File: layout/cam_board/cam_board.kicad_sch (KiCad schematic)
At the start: 46 parts, among them J1 Debug, J2 USB Connector, J3 BATT_CONNECTOR, SW1 SW_MEC_5E, SW2 SW_MEC_5E, SW3 SW_MEC_5E, SW4 PWR, U1 STM32F401CCUx, U2 USBLC6-2SC6, U3 LD1117S33TR_SOT223, U4 MCP73831-2-OT, Y1 ECS-80-18-23B-JTN-TR, Y2 SC32S-7PF20PPM

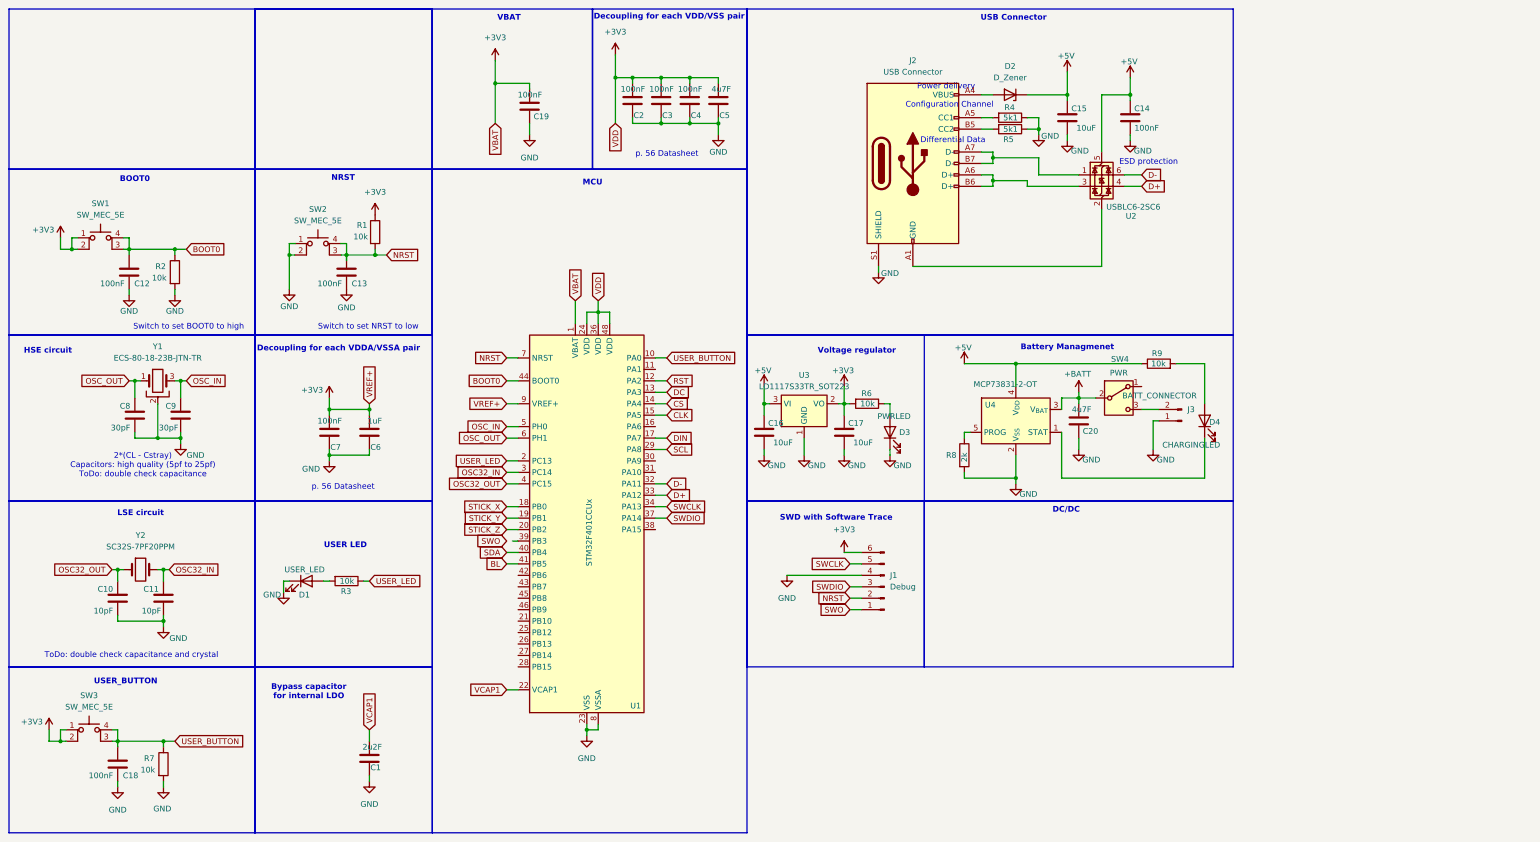
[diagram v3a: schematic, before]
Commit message: Update layout and schematic
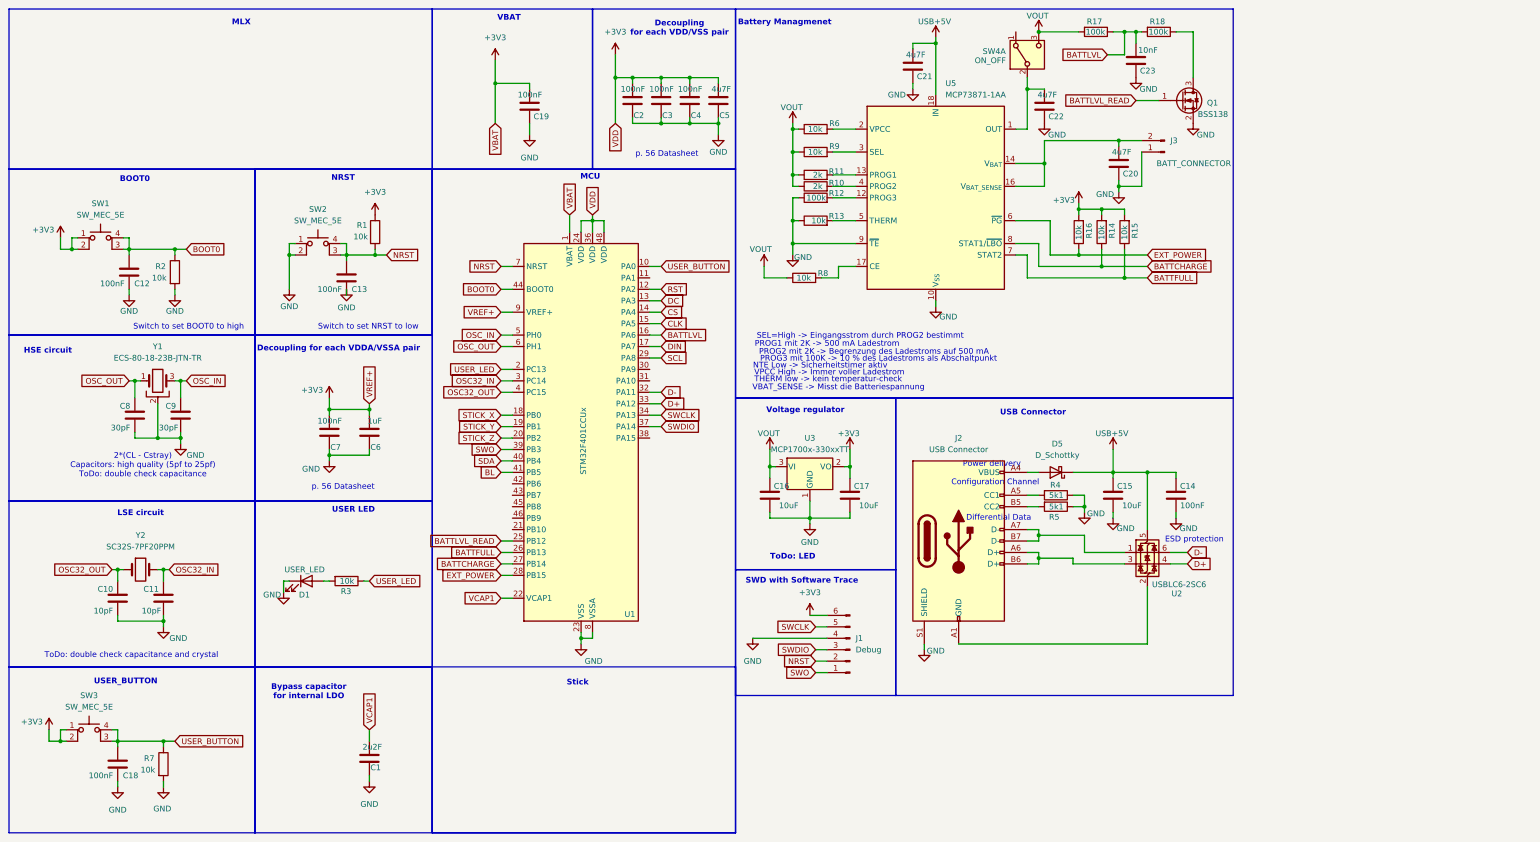
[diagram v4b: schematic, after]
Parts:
- removed D2: D_Zener, Diode_SMD:D_0201_0603Metric_Pad0.64x0.40mm_HandSolder, symbol Device:D_Zener
- removed D3: PWRLED, LED_SMD:LED_0603_1608Metric_Pad1.05x0.95mm_HandSolder, symbol Device:LED
- removed D4: CHARGINGLED, LED_SMD:LED_0603_1608Metric_Pad1.05x0.95mm_HandSolder, symbol Device:LED
- removed SW4: PWR, symbol Switch:SW_SPDT
- removed U3: LD1117S33TR_SOT223, Package_TO_SOT_SMD:SOT-223-3_TabPin2, symbol Regulator_Linear:LD1117S33TR_SOT223
- removed U4: MCP73831-2-OT, Package_TO_SOT_SMD:SOT-23-5_HandSoldering, symbol Battery_Management:MCP73831-2-OT
- added C21, C22: 4u7F, Capacitor_SMD:C_0603_1608Metric_Pad1.08x0.95mm_HandSolder, symbol Device:C
- added C23: 10nF, Capacitor_SMD:C_0603_1608Metric_Pad1.08x0.95mm_HandSolder, symbol Device:C
- added D5: D_Schottky, Diode_SMD:D_0603_1608Metric_Pad1.05x0.95mm_HandSolder, symbol Device:D_Schottky
- added Q1: BSS138, Package_TO_SOT_SMD:SOT-23_Handsoldering, symbol Transistor_FET:BSS138
- added R10, R11: 2k, Resistor_SMD:R_0603_1608Metric_Pad0.98x0.95mm_HandSolder, symbol Device:R
- added R12, R17, R18: 100k, Resistor_SMD:R_0603_1608Metric_Pad0.98x0.95mm_HandSolder, symbol Device:R
- added R13, R14, R15, R16: 10k, Resistor_SMD:R_0603_1608Metric_Pad0.98x0.95mm_HandSolder, symbol Device:R
- added SW4: ON_OFF, symbol Switch:SW_DPDT_x2
- added U3: MCP1700x-330xxTT, Package_TO_SOT_SMD:SOT-23_Handsoldering, symbol Regulator_Linear:MCP1700x-330xxTT
- added U5: MCP73871-1AA, Package_DFN_QFN:QFN-20-1EP_4x4mm_P0.5mm_EP2.5x2.5mm_ThermalVias, symbol Battery_Management:MCP73871-1AA
- R8: value 2k -> 10k
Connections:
- net +BATT is gone; now on an unnamed net: C20.2
- net +3V3: now also R14.2, R15.2, R16.2, U3.2 (VO); no longer R6.2
- net GND: now also C21.1, C22.1, C23.1, Q1.2 (S), R12.1, R13.1, U3.1 (GND), U5.10 (V_{SS}), U5.11 (V_{SS}), U5.21 (V_{SS}), U5.9 (~{TE}); no longer R8.2
- net SWO: now also U1.39 (PB3)
- net at R9.2: now also U5.3 (SEL)
- net at J3.2 (Pin_2): now also U5.14 (V_{BAT}), U5.15 (V_{BAT}), U5.16 (V_{BAT_SENSE})
- net at J2.A4 (VBUS), J2.A9 (VBUS), J2.B4 (VBUS)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: now also D5.2 (A)
- net BATTLVL: now reaches U1.16 (PA6)
- net BATTLVL: now also C23.2, R17.1, R18.2
- net BATTLVL_READ: now reaches U1.25 (PB12)
- net BATTLVL_READ: now also Q1.1 (G)
- net BATTFULL: now reaches U1.26 (PB13)
- net BATTFULL: now also R15.1, U5.7 (STAT2)
- net BATTCHARGE: now reaches U1.27 (PB14)
- net BATTCHARGE: now also R14.1, U5.8 (STAT1/~{LBO})
- net EXT_POWER: now reaches U1.28 (PB15)
- net EXT_POWER: now also R16.1, U5.6 (~{PG})
- net VOUT: now reaches R8.1
- net VOUT: now also C16.2, R6.1, R9.1, R10.1, R11.1, R17.2, SW4.3 (C), U3.3 (VI)
- net +5V renamed USB+5V
- net USB+5V: now also C21.2, D5.1 (K), U5.18 (IN), U5.19 (IN); no longer C16.2, R9.1
- new net: R10.2, U5.4 (PROG2)
- new net: R6.2, U5.2 (VPCC)
- new net: R11.2, U5.13 (PROG1)
- new net: R13.2, U5.5 (THERM)
- new net: C22.2, SW4.2 (B), U5.1 (OUT), U5.20 (OUT)
- new net: Q1.3 (D), R18.1
- new net: R12.2, U5.12 (PROG3)
- new net: R8.2, U5.17 (CE)
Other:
- note added: "MLX"
- note added: "NTE Low -> Sicherheitstimer aktiv"
- note added: "PROG1 mit 2K -> 500 mA Ladestrom"
- note added: "PROG2 mit 2K -> Begrenzung des Ladestroms auf 500 mA"
- note added: "PROG3 mit 100K -> 10 % des Ladestroms als Abschaltpunkt"
- note added: "SEL=High -> Eingangsstrom durch PROG2 bestimmt"
- note added: "Stick"
- note added: "THERM low -> kein temperatur-check"
- note added: "ToDo: LED"
- note added: "VBAT_SENSE -> Misst die Batteriespannung"
- note added: "VPCC High -> Immer voller Ladestrom"
- note removed: "DC/DC"
- moved on the sheet: C13, C14, C15, C16, C17, C20, J1, J2, J3, R4, R5, U1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

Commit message: First full schematic
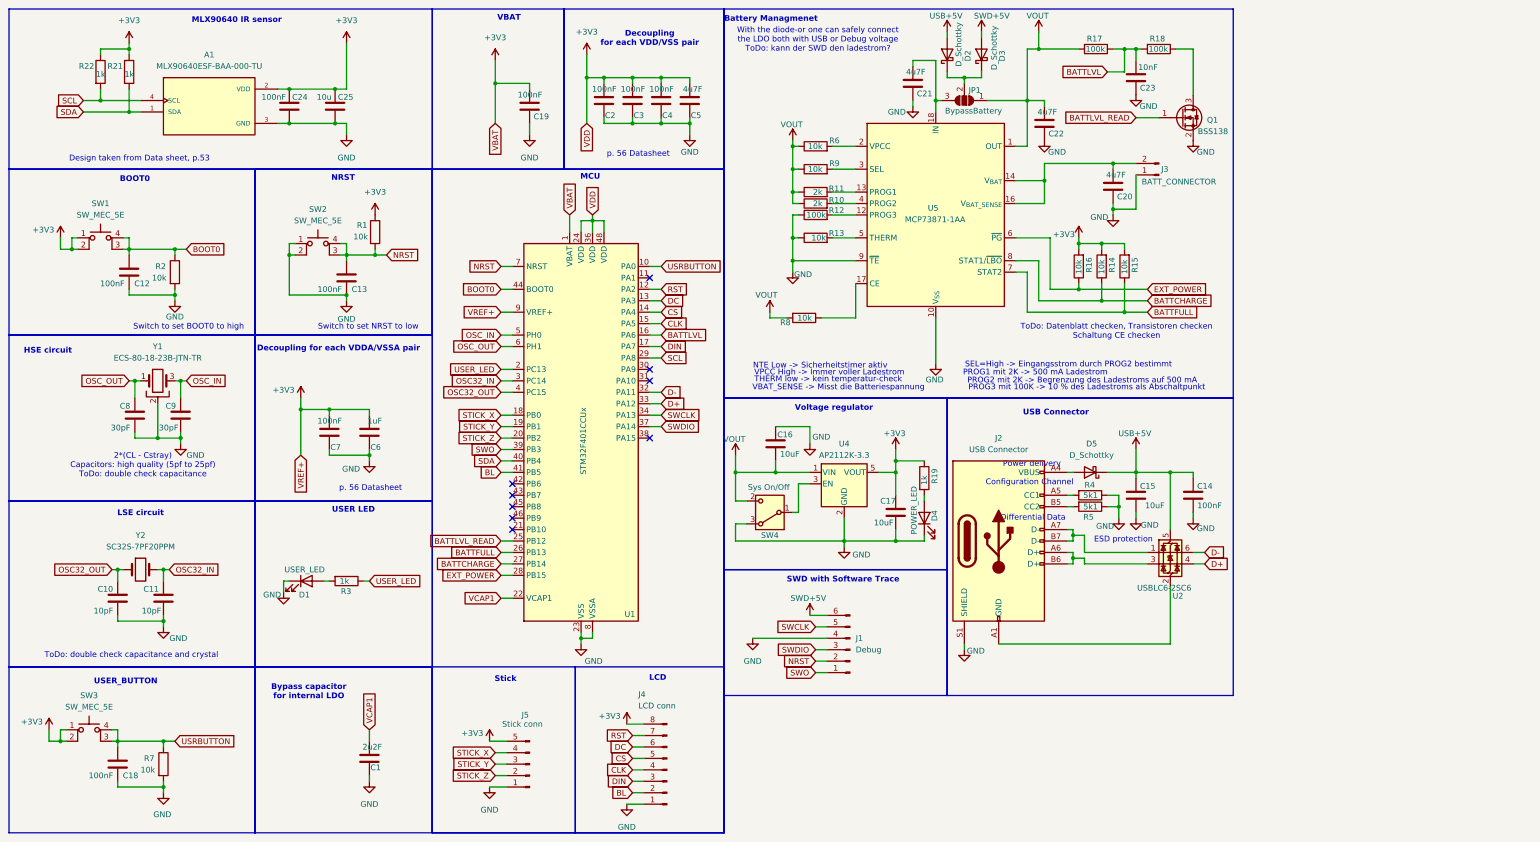
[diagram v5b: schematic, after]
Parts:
- removed SW4: ON_OFF, symbol Switch:SW_DPDT_x2
- removed U3: MCP1700x-330xxTT, Package_TO_SOT_SMD:SOT-23_Handsoldering, symbol Regulator_Linear:MCP1700x-330xxTT
- added A1: MLX90640ESF-BAA-000-TU, A_Custom:TO292P930H600-4-MLX, symbol Custom:MLX90640ESF-BAA-000-TU
- added C24: 100nF, Capacitor_SMD:C_0603_1608Metric_Pad1.08x0.95mm_HandSolder, symbol Device:C
- added C25: 10u, Capacitor_SMD:C_0603_1608Metric_Pad1.08x0.95mm_HandSolder, symbol Device:C
- added D2, D3: D_Schottky, Diode_SMD:D_0603_1608Metric_Pad1.05x0.95mm_HandSolder, symbol Device:D_Schottky
- added D4: POWER_LED, LED_SMD:LED_0603_1608Metric_Pad1.05x0.95mm_HandSolder, symbol Device:LED
- added J4: LCD conn, Connector_PinHeader_1.27mm:PinHeader_1x08_P1.27mm_Vertical, symbol Connector:Conn_01x08_Pin
- added J5: Stick conn, Connector_PinHeader_1.27mm:PinHeader_1x05_P1.27mm_Vertical, symbol Connector:Conn_01x05_Pin
- added JP1: BypassBattery, Jumper:SolderJumper-3_P1.3mm_Open_RoundedPad1.0x1.5mm_NumberLabels, symbol Jumper:SolderJumper_3_Open
- added R19, R21, R22: 1k, Resistor_SMD:R_0603_1608Metric_Pad0.98x0.95mm_HandSolder, symbol Device:R
- added SW4: Sys On/Off, Button_Switch_SMD:SW_DIP_SPSTx01_Slide_6.7x4.1mm_W6.73mm_P2.54mm_LowProfile_JPin, symbol Switch:SW_SPDT_312
- added U4: AP2112K-3.3, Package_TO_SOT_SMD:SOT-23-5_HandSoldering, symbol Regulator_Linear:AP2112K-3.3
- J1: footprint (none) -> Connector_PinHeader_1.27mm:PinHeader_1x06_P1.27mm_Vertical
- J2: footprint (none) -> Connector_USB:USB_C_Receptacle_HRO_TYPE-C-31-M-12
- J3: footprint (none) -> Connector_JST:JST_PH_B2B-PH-K_1x02_P2.00mm_Vertical
- R3: value 10k -> 1k
- Y1: footprint (none) -> A_Custom:XTAL_ECS-80-18-23B-JTN-TR
- Y2: footprint (none) -> A_Custom:XTAL_CM8V-T1A-32.768KHZ-6PF-20PPM-TA-QC
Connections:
- net +3V3: now also A1.2 (VDD), C24.2, C25.2, J4.8 (Pin_8), J5.5 (Pin_5), R19.1, R21.1, R22.1, U4.5 (VOUT); no longer J1.6 (Pin_6)
- net BL: now also J4.2 (Pin_2)
- net CLK: now also J4.4 (Pin_4)
- net CS: now also J4.5 (Pin_5)
- net DC: now also J4.6 (Pin_6)
- net DIN: now also J4.3 (Pin_3)
- net GND: now also C16.2, A1.3 (GND), C24.1, C25.1, D4.1 (K), J4.1 (Pin_1), J5.1 (Pin_1), SW4.3 (A), U4.2 (GND); no longer C16.1
- net RST: now also J4.7 (Pin_7)
- net SCL: now also A1.4 (SCL), R22.2
- net SDA: now also A1.1 (SDA), R21.2
- net STICK_X: now also J5.4 (Pin_4)
- net STICK_Y: now also J5.3 (Pin_3)
- net STICK_Z: now also J5.2 (Pin_2)
- net USB+5V: now also D2.2 (A); no longer C21.2, U5.18 (IN), U5.19 (IN)
- net VOUT: now also C16.1, C22.2, R8.2, U5.1 (OUT), U5.20 (OUT), JP1.1 (A), SW4.2 (C), U4.1 (VIN); no longer C16.2, R8.1
- net at U5.17 (CE): now also R8.1; no longer R8.2
- net USER_BUTTON renamed USRBUTTON
- new net: D2.1 (K), D3.1 (K), JP1.2 (C)
- new net: C21.2, JP1.3 (B), U5.18 (IN), U5.19 (IN)
- new net: D4.2 (A), R19.2
- new net: SW4.1 (B), U4.3 (EN)
- new net SWD+5V: D3.2 (A), J1.6 (Pin_6)
- no-connect marks 0 -> 9
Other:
- note added: "Design taken from Data sheet, p.53"
- note added: "LCD"
- note added: "MLX90640 IR sensor"
- note added: "ToDo: Datenblatt checken, Transistoren checken Schaltung CE checken"
- note added: "With the diode-or one can safely connect the LDO both with USB or Debug voltage ToDo: kann der SWD den ladestrom?"
- note removed: "MLX"
- note removed: "ToDo: LED"
- moved on the sheet: C14, C15, C16, C17, C2, C20, C21, C22, C23, C3, C4, C5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

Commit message: Update layout and schematic
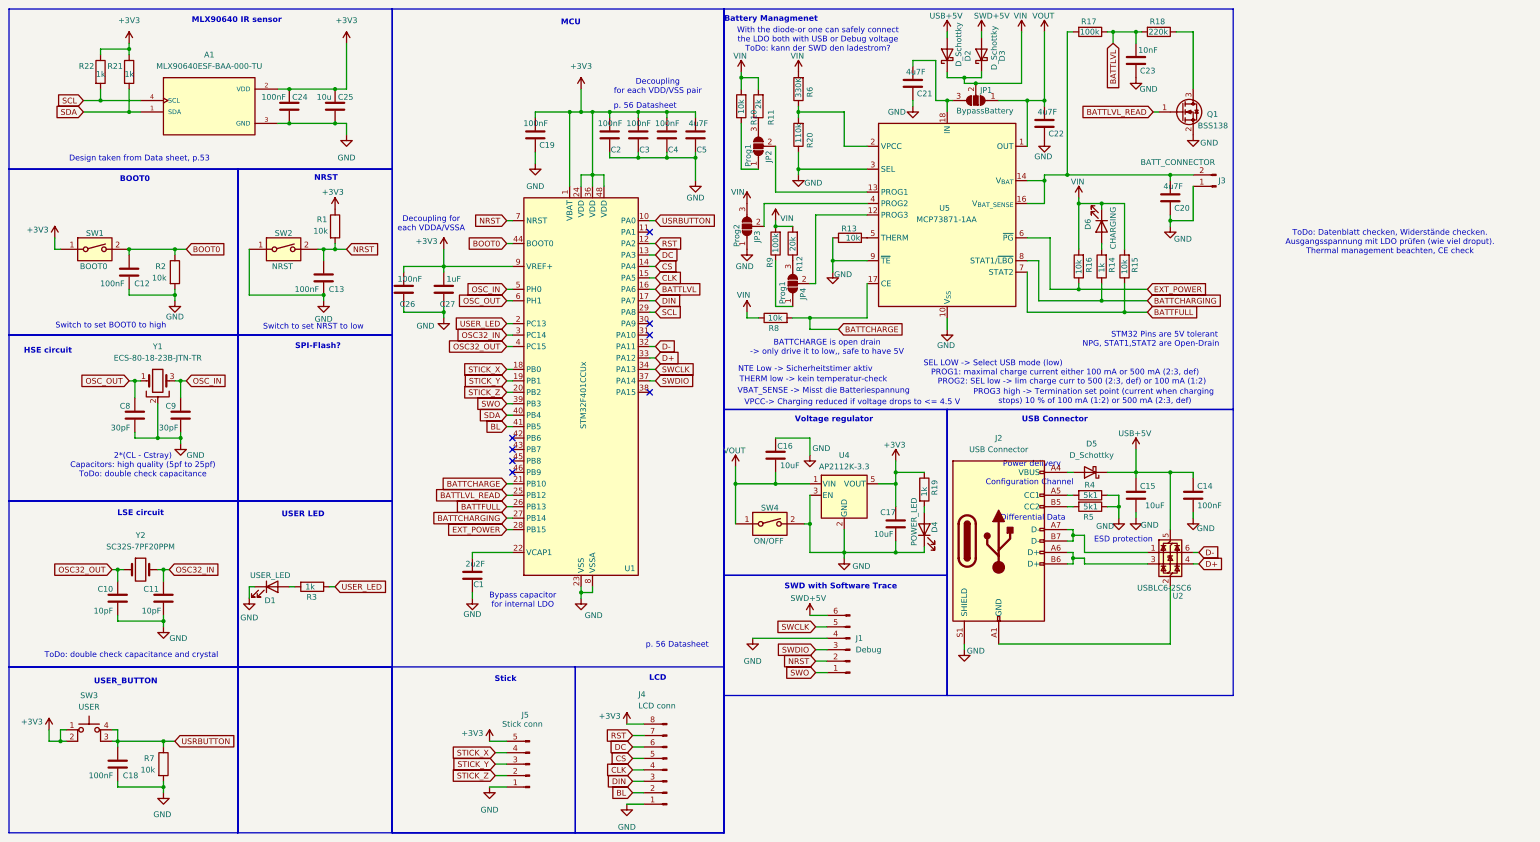
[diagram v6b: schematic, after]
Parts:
- removed C6: 1uF, Capacitor_SMD:C_0603_1608Metric_Pad1.08x0.95mm_HandSolder, symbol Device:C
- removed C7: 100nF, Capacitor_SMD:C_0603_1608Metric_Pad1.08x0.95mm_HandSolder, symbol Device:C
- removed SW1, SW2: SW_MEC_5E, Button_Switch_SMD:SW_MEC_5GSH9, symbol Switch:SW_MEC_5E
- removed SW4: Sys On/Off, Button_Switch_SMD:SW_DIP_SPSTx01_Slide_6.7x4.1mm_W6.73mm_P2.54mm_LowProfile_JPin, symbol Switch:SW_SPDT_312
- added C26: 100nF, Capacitor_SMD:C_0402_1005Metric_Pad0.74x0.62mm_HandSolder, symbol Device:C
- added C27: 1uF, Capacitor_SMD:C_0402_1005Metric_Pad0.74x0.62mm_HandSolder, symbol Device:C
- added D6: CHARGING, LED_SMD:LED_0603_1608Metric_Pad1.05x0.95mm_HandSolder, symbol Device:LED
- added JP2, JP4: Prog1, Jumper:SolderJumper-3_P1.3mm_Open_RoundedPad1.0x1.5mm_NumberLabels, symbol Jumper:SolderJumper_3_Open
- added JP3: Prog2, Jumper:SolderJumper-3_P1.3mm_Open_RoundedPad1.0x1.5mm_NumberLabels, symbol Jumper:SolderJumper_3_Open
- added R20: 110k, Resistor_SMD:R_0603_1608Metric_Pad0.98x0.95mm_HandSolder, symbol Device:R
- added SW1: BOOT0, Button_Switch_SMD:SW_DIP_SPSTx01_Slide_9.78x4.72mm_W8.61mm_P2.54mm, symbol Switch:SW_DIP_x01
- added SW2: NRST, Button_Switch_SMD:SW_DIP_SPSTx01_Slide_9.78x4.72mm_W8.61mm_P2.54mm, symbol Switch:SW_DIP_x01
- added SW4: ON/OFF, Button_Switch_SMD:SW_DIP_SPSTx01_Slide_9.78x4.72mm_W8.61mm_P2.54mm, symbol Switch:SW_DIP_x01
- C1, C10, C11, C19, C2, C3, C4, C5, C8, C9: footprint Capacitor_SMD:C_0603_1608Metric_Pad1.08x0.95mm_HandSolder -> Capacitor_SMD:C_0402_1005Metric_Pad0.74x0.62mm_HandSolder
- R10: value 2k -> 10k
- R12: value 100k -> 20k
- R14: value 10k -> 1k
- R18: value 100k -> 220k
- R6: value 10k -> 330K
- R9: value 10k -> 100k
- SW3: value SW_MEC_5E -> USER; footprint Button_Switch_SMD:SW_MEC_5GSH9 -> A_Custom:SW_1825910-6-4
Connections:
- net +3V3: now also C26.2, C27.2, SW1.1; no longer R14.2, R15.2, R16.2
- net BATTCHARGE: now also R8.2, U1.21 (PB10), U5.17 (CE); no longer R14.1, U1.27 (PB14), U5.8 (STAT1/~{LBO})
- net BOOT0: now also SW1.2
- net GND: now also U4.3 (EN), U5.3 (SEL), C26.1, C27.1, JP3.1 (A), R20.1, SW2.1, SW4.2; no longer R12.1
- net NRST: now also SW2.2
- net VOUT: now also SW4.1; no longer R10.1, R11.1, R17.2, R6.1, R8.2, R9.1
- net at U5.4 (PROG2): now also JP3.2 (C); no longer R10.2
- net at C20.2, J3.2 (Pin_2), U5.14 (V_{BAT})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: now also R17.2
- net at U5.2 (VPCC): now also R6.1, R20.2; no longer R6.2
- net VIN: now reaches D2.1 (K), D3.1 (K), JP1.2 (C)
- net VIN: now also R10.2, R11.2, R12.2, R15.2, R16.2, R6.2, R8.1, R9.2, D6.1 (K), JP3.3 (B)
- net at U5.13 (PROG1): now also JP2.2 (C); no longer R11.2
- net at U5.12 (PROG3): now also JP4.2 (C); no longer R12.2
- net VCAP1: no longer names the net of C1.2, U1.22 (VCAP1)
- new net: JP4.1 (A), R9.1
- new net: JP2.3 (B), R11.1
- new net: JP2.1 (A), R10.1
- new net: JP4.3 (B), R12.1
- new net: D6.2 (A), R14.2
- new net BATTCHARGING: R14.1, U1.27 (PB14), U5.8 (STAT1/~{LBO})
- no-connect marks 9 -> 8
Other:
- note added: "BATTCHARGE is open drain -> only drive it to low,, safe to have 5V"
- note added: "Decoupling for each VDDA/VSSA"
- note added: "NPG, STAT1,STAT2 are Open-Drain"
- note added: "PROG1: maximal charge current either 100 mA or 500 mA (2:3, def)"
- note added: "PROG2: SEL low -> lim charge curr to 500 (2:3, def) or 100 mA (1:2)"
- note added: "PROG3 high -> Termination set point (current when charging stops) 10 % of 100 mA (1:2) or 500 mA (2:3, def)"
- note added: "SEL LOW -> Select USB mode (low)"
- note added: "SPI-Flash?"
- note added: "STM32 Pins are 5V tolerant"
- note added: "ToDo: Datenblatt checken, Widerstände checken. Ausgangsspannung mit LDO prüfen (wie viel droput). Thermal management beachten, CE check"
- note added: "VPCC-> Charging reduced if voltage drops to <= 4.5 V"
- note removed: "Decoupling for each VDDA/VSSA pair"
- note removed: "PROG1 mit 2K -> 500 mA Ladestrom"
- note removed: "PROG2 mit 2K -> Begrenzung des Ladestroms auf 500 mA"
- note removed: "PROG3 mit 100K -> 10 % des Ladestroms als Abschaltpunkt"
- note removed: "SEL=High -> Eingangsstrom durch PROG2 bestimmt"
- note removed: "ToDo: Datenblatt checken, Transistoren checken Schaltung CE checken"
- note removed: "VBAT"
- note removed: "VPCC High -> Immer voller Ladestrom"
- moved on the sheet: C1, C13, C16, C17, C19, C2, C20, C23, C3, C4, C5, D1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
